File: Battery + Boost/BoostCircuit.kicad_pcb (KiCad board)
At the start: 2 copper layers, 30 x 30 mm, 7 parts, among them J1 Conn_01x04_Pin, J2 Conn_01x04_Pin, U1 TPS610995DRVR

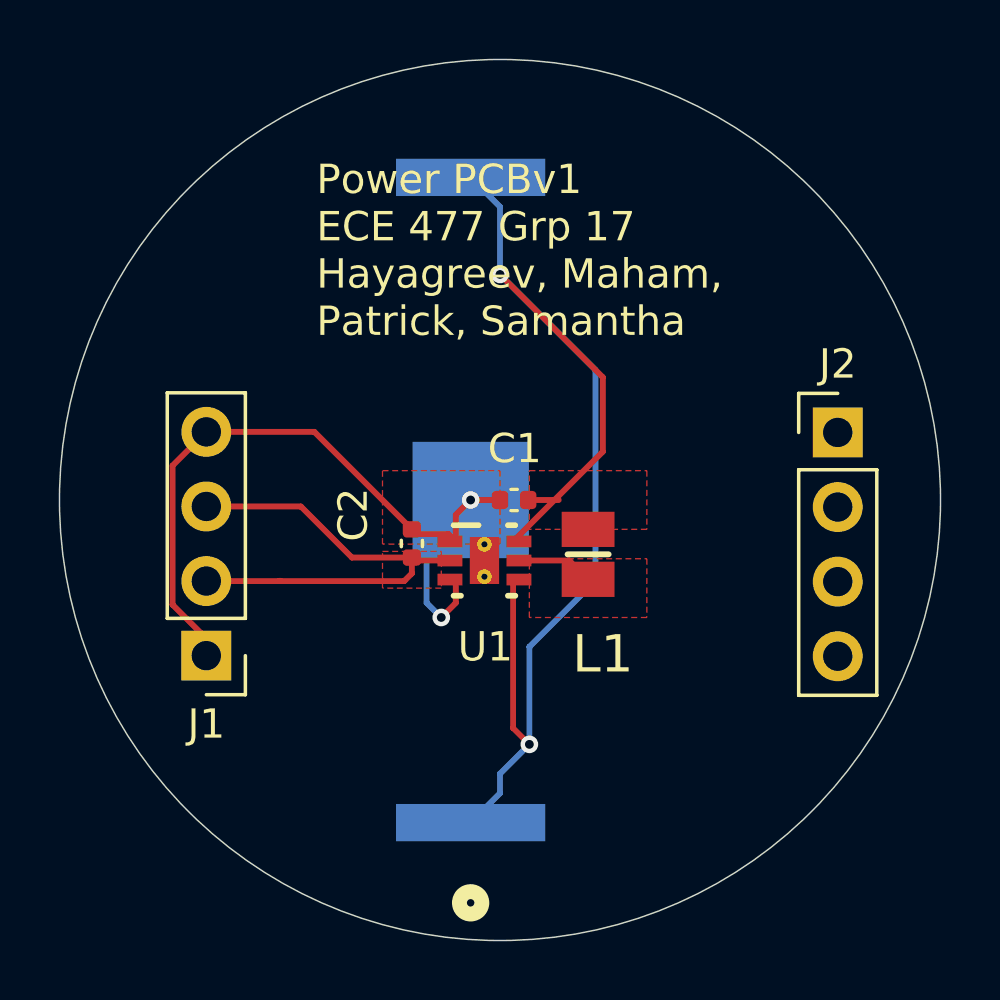
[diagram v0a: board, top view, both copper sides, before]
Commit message: final
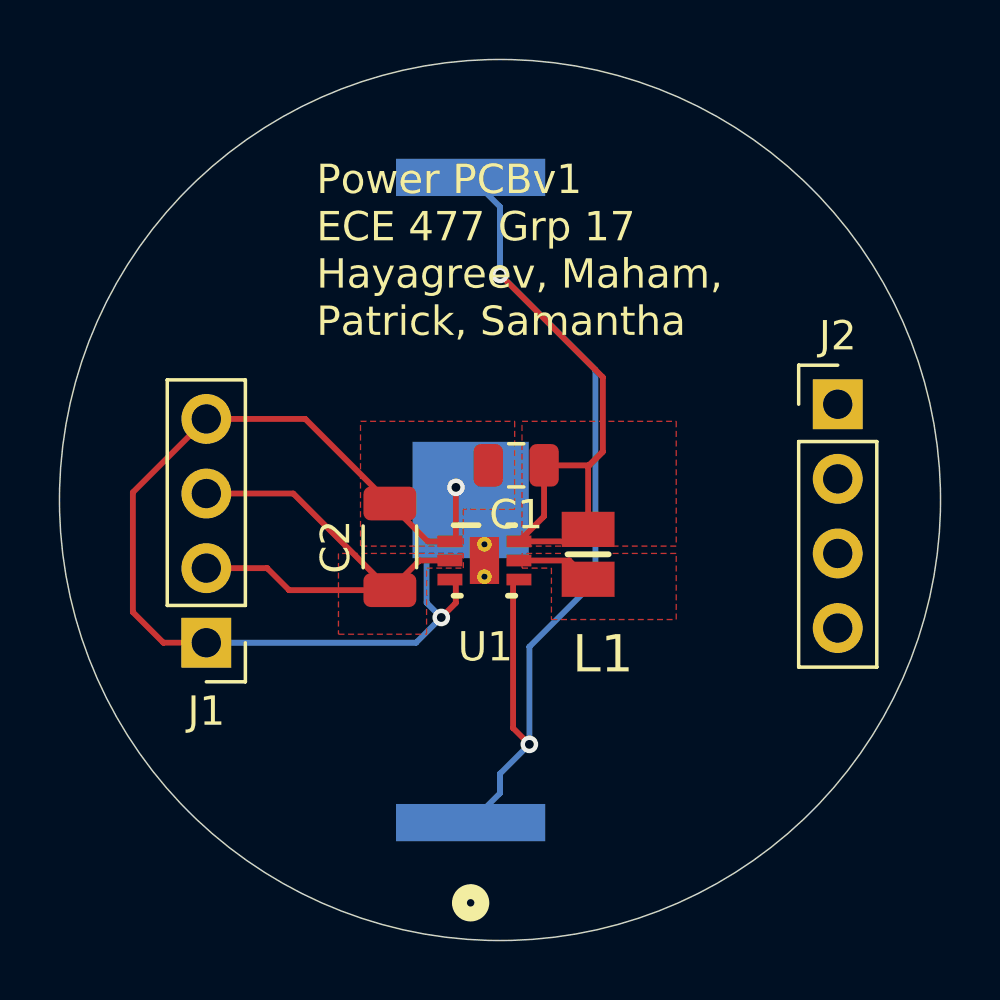
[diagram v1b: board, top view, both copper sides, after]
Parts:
- C1: footprint Capacitor_SMD:C_0402_1005Metric -> Capacitor_SMD:C_0805_2012Metric
- C2: footprint Capacitor_SMD:C_0402_1005Metric -> Capacitor_SMD:C_1206_3216Metric
- moved C1 1.18 mm to (133.1, 101.2)
- moved J2 0.96 mm to (144.0, 99.2)
- moved C2 0.76 mm to (128.8, 104.0)
- moved J1 0.44 mm to (122.5, 107.3)
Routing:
- net GND: track 27.5 -> 37.9 mm
- net Net-(U1-EN): track 44.2 -> 49.3 mm
